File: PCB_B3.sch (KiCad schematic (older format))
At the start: 18 parts, among them P1 Digital, P3 ADC, P4 Analog, P5 ADC

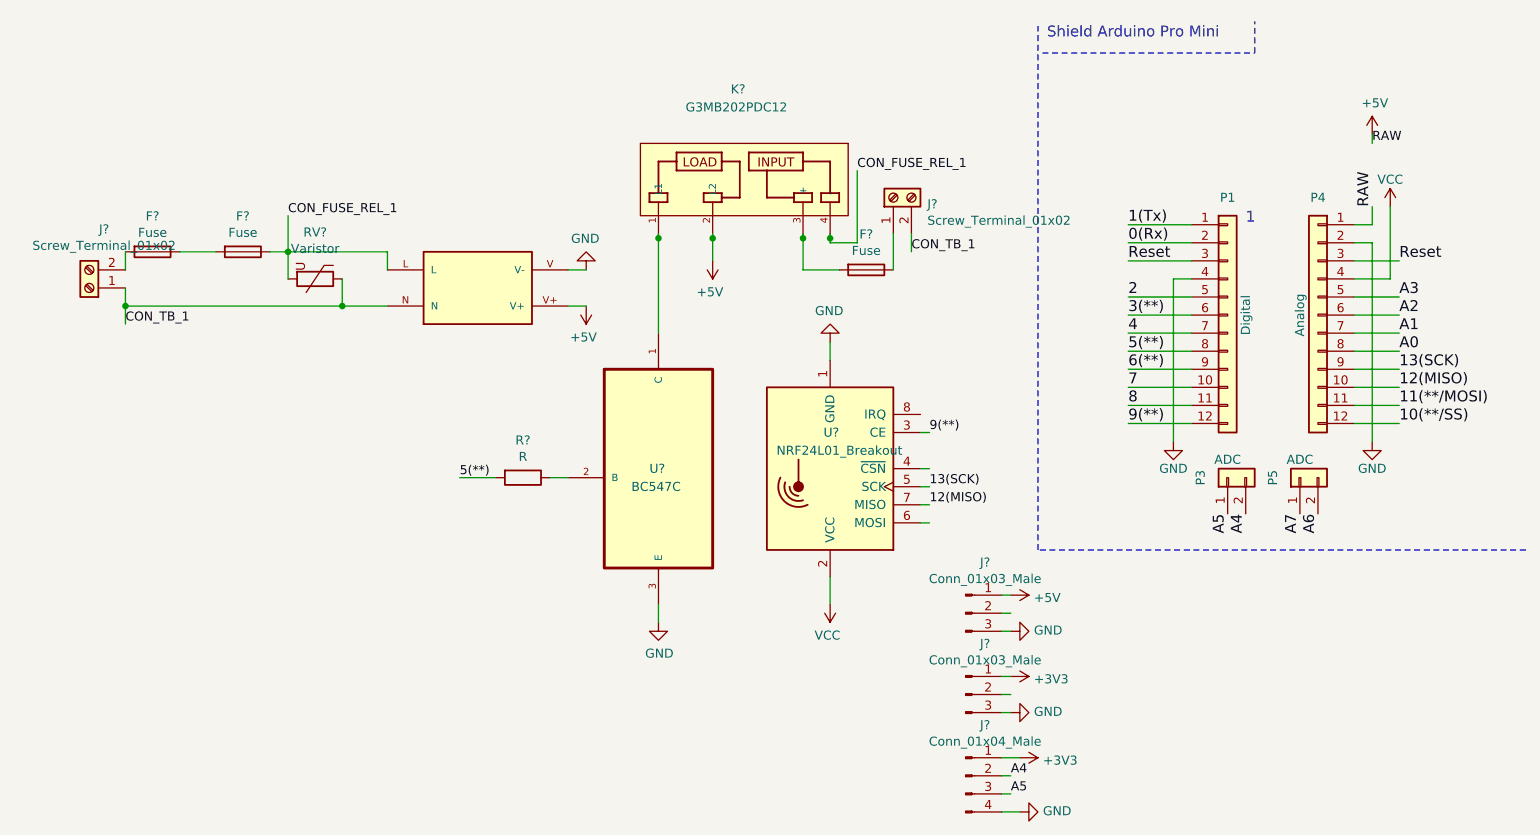
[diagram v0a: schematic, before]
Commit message: Update
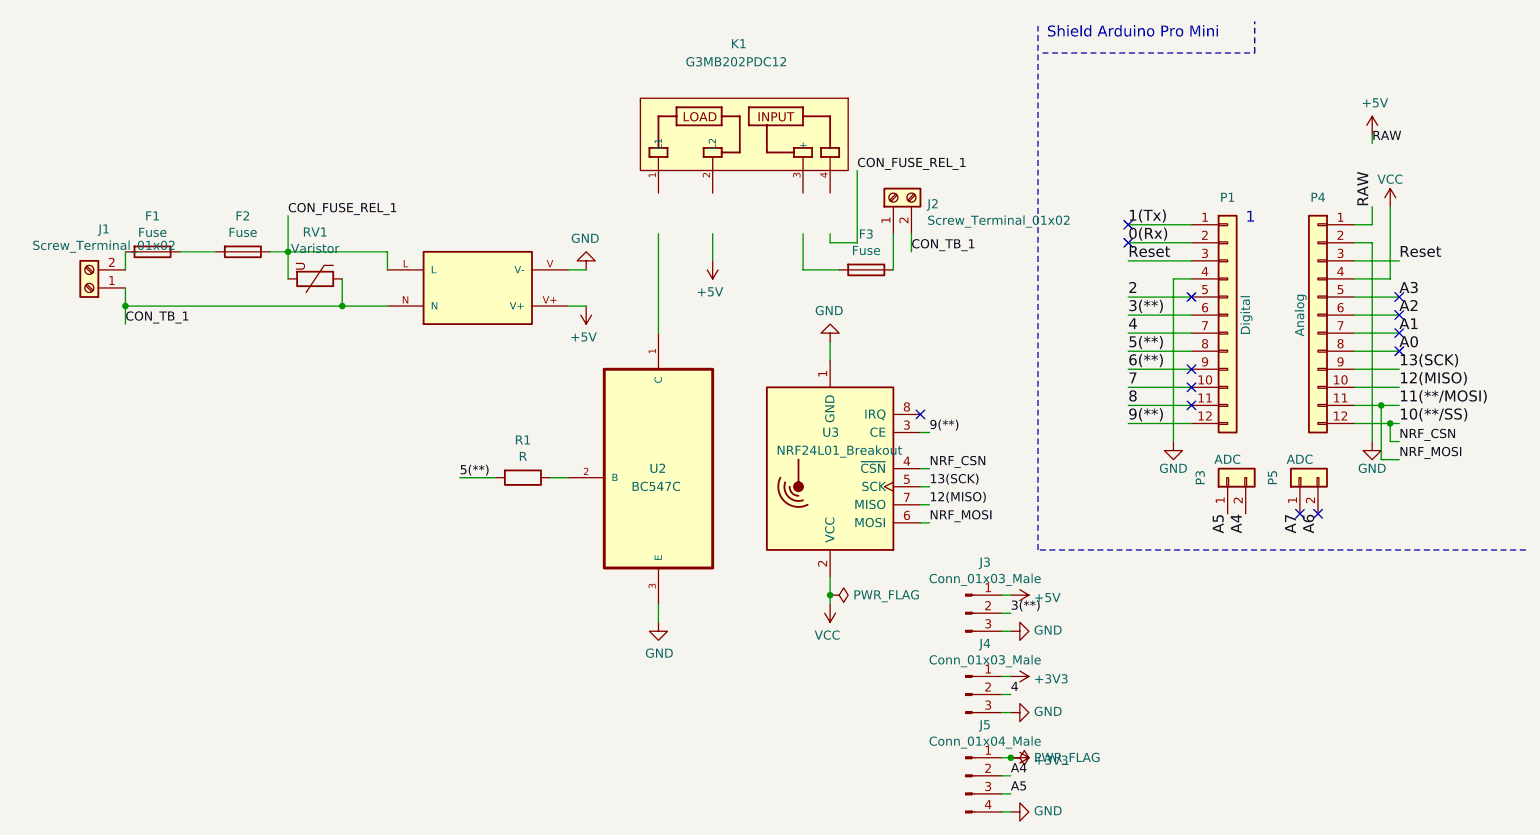
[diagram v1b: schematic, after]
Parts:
- F1, F2, F3: renamed from F?; footprint (none) -> Resistor_THT:R_Axial_DIN0414_L11.9mm_D4.5mm_P15.24mm_Horizontal
- J1, J2: renamed from J?; footprint (none) -> TerminalBlock:TerminalBlock_Altech_AK300-2_P5.00mm
- J3, J4: renamed from J?; footprint (none) -> Connector_PinHeader_2.54mm:PinHeader_1x03_P2.54mm_Vertical
- J5: renamed from J?; footprint (none) -> Connector_PinHeader_2.54mm:PinHeader_1x04_P2.54mm_Vertical
- K1: renamed from K?; footprint RELAY_G3MB202PDC12 -> footprints_externos:RELAY_G3MB202PDC12
- R1: renamed from R?; footprint (none) -> Resistor_SMD:R_1206_3216Metric_Pad1.30x1.75mm_HandSolder
- RV1: renamed from RV?; footprint (none) -> Varistor:RV_Disc_D12mm_W6.2mm_P7.5mm
- U1: renamed from U?; footprint HLK-PM01-PAK -> Converter_ACDC:Converter_ACDC_HiLink_HLK-PMxx
- U2: renamed from U?; footprint TO127P254X732-3 -> footprints_externos:BC547C
- gave numbers to parts that had none: 1
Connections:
- net labels added: NRF_CSN, NRF_MOSI
- wire segments 76 -> 79
- no-connect marks 0 -> 13
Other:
- moved on the sheet: K1

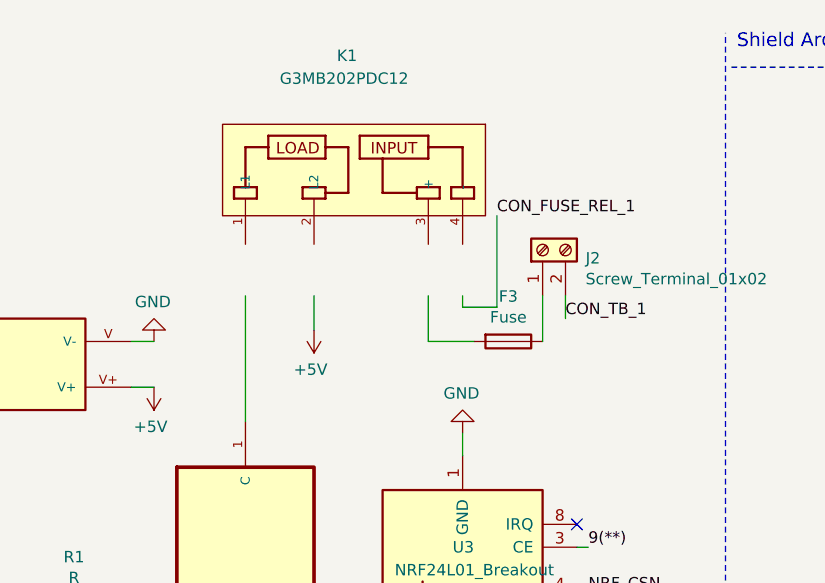
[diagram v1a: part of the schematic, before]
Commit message: Update
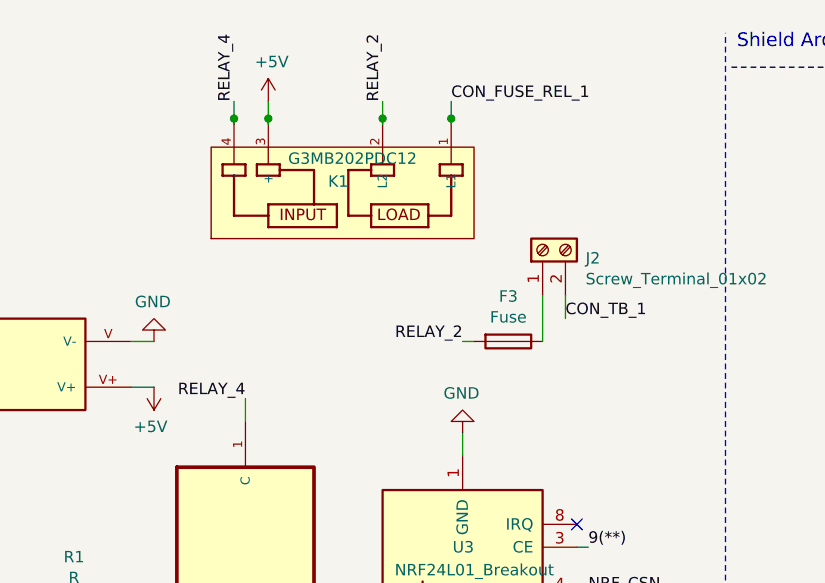
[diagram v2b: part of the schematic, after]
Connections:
- net labels added: RELAY_2, RELAY_4
- wire segments 79 -> 82
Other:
- moved on the sheet: K1
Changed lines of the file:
@@
 L simbolos_externos:G3MB202PDC12 K1
 U 1 1 60094688
-P 6850 1100
-F 0 "K1" H 6900 600 50  0000 R CNN
-F 1 "G3MB202PDC12" H 7150 700 50  0000 R CNN
-F 2 "footprints_externos:RELAY_G3MB202PDC12" H 6850 1100 50  0001 L BNN
-F 3 "" H 6850 1100 50  0001 L BNN
-F 4 "N/A" H 6850 1100 50  0001 L BNN "PARTREV"
-F 5 "Omron" H 6850 1100 50  0001 L BNN "MANUFACTURER"
-F 6 "Manufacturer Recommendation" H 6850 1100 50  0001 L BNN "STANDARD"
-	1    6850 1100
-	-1   0    0    1
+P 6850 1200
+F 0 "K1" H 6850 1250 50  0000 R CNN
+F 1 "G3MB202PDC12" H 7150 1350 50  0000 R CNN
+F 2 "footprints_externos:RELAY_G3MB202PDC12" H 6850 1200 50  0001 L BNN
+F 3 "" H 6850 1200 50  0001 L BNN
+F 4 "N/A" H 6850 1200 50  0001 L BNN "PARTREV"
+F 5 "Omron" H 6850 1200 50  0001 L BNN "MANUFACTURER"
+F 6 "Manufacturer Recommendation" H 6850 1200 50  0001 L BNN "STANDARD"
+	1    6850 1200
+	1    0    0    -1
 $EndComp
 $Comp
@@
 L power:+5V #PWR07
 U 1 1 600AA64D
-P 6700 1800
-F 0 "#PWR07" H 6700 1650 50  0001 C CNN
-F 1 "+5V" H 6715 1973 50  0000 C CNN
-F 2 "" H 6700 1800 50  0001 C CNN
-F 3 "" H 6700 1800 50  0001 C CNN
-	1    6700 1800
-	-1   0    0    1
-$EndComp
-Wire Wire Line
-	7200 1850 7400 1850
+P 6500 800
+F 0 "#PWR07" H 6500 650 50  0001 C CNN
+F 1 "+5V" H 6515 973 50  0000 C CNN
+F 2 "" H 6500 800 50  0001 C CNN
+F 3 "" H 6500 800 50  0001 C CNN
+	1    6500 800
+	1    0    0    -1
+$EndComp
 Wire Wire Line
 	7700 1850 7700 1650
@@
 Text Label 4350 1550 0    50   ~ 0
 CON_FUSE_REL_1
-Text Label 7500 1300 0    50   ~ 0
+Text Label 7300 800  0    50   ~ 0
 CON_FUSE_REL_1
-Wire Wire Line
-	7500 1700 7500 1300
-Wire Wire Line
-	7350 1700 7500 1700
 Wire Wire Line
 	3450 2050 3450 2150
@@
 	0    -1   -1   0
 $EndComp
-$Comp
-L power:+3V3 #PWR014
-U 1 1 60109C1C
-P 8350 4550
-F 0 "#PWR014" H 8350 4400 50  0001 C CNN
-F 1 "+3V3" V 8365 4678 50  0000 L CNN
-F 2 "" H 8350 4550 50  0001 C CNN
-F 3 "" H 8350 4550 50  0001 C CNN
-	1    8350 4550
-	0    1    1    0
-$EndComp
-Wire Wire Line
-	8300 4550 8350 4550
 Wire Wire Line
 	8300 4850 8350 4850
@@
 Wire Wire Line
 	7350 3650 7350 3550
+Text Label 6350 800  1    50   ~ 0
+RELAY_4
+Text Label 7000 800  1    50   ~ 0
+RELAY_2
+Text Label 6400 2100 2    50   ~ 0
+RELAY_4
+Text Label 7350 1850 2    50   ~ 0
+RELAY_2
+Wire Wire Line
+	7400 1850 7350 1850
+Wire Wire Line
+	7300 800  7300 875
+Connection ~ 7300 875
+Wire Wire Line
+	7300 875  7300 900
+Wire Wire Line
+	7000 800  7000 875
+Connection ~ 7000 875
+Wire Wire Line
+	7000 875  7000 900
+Connection ~ 8350 4550
+Wire Wire Line
+	8300 4550 8350 4550
+$Comp
+L power:+3V3 #PWR014
+U 1 1 60109C1C
+P 8350 4550
+F 0 "#PWR014" H 8350 4400 50  0001 C CNN
+F 1 "+3V3" V 8365 4678 50  0000 L CNN
+F 2 "" H 8350 4550 50  0001 C CNN
+F 3 "" H 8350 4550 50  0001 C CNN
+	1    8350 4550
+	0    1    1    0
+$EndComp
 $Comp
 L power:PWR_FLAG #FLG0102
@@
 	0    1    1    0
 $EndComp
-Connection ~ 8350 4550
-Wire Wire Line
-	6700 1650 6700 1800
-Wire Wire Line
-	7200 1650 7200 1850
-Wire Wire Line
-	7350 1650 7350 1700
-Wire Wire Line
-	6400 1650 6400 2200
+Wire Wire Line
+	6350 800  6350 875
+Wire Wire Line
+	6350 875  6350 900
+Connection ~ 6350 875
+Wire Wire Line
+	6400 2200 6400 2100
+Wire Wire Line
+	6500 800  6500 875
+Connection ~ 6500 875
+Wire Wire Line
+	6500 875  6500 900
 $EndSCHEMATC
